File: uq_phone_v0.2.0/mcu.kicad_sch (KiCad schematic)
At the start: 23 parts, among them J6 Conn_ARM_SWD_TagConnect_TC2030, U5 TXB0108YZPR2, U6 STM32H733VGHx, U7 TXB0108YZPR2

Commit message: New Layout
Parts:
- removed R21: 4.7k, Resistor_SMD:R_0201_0603Metric, symbol Resistors:Resistor_4k7
- removed U5: TXB0108YZPR2, TXB0108YZPR2:YZP20, symbol TXB0108YZPR2:TXB0108YZPR2
- added C50, C51: 100nF, Capacitor_SMD:C_0201_0603Metric, symbol Capacitors:capacitor_100nF
- added J7, J9: 559092474, 559092474:CON_559092474, symbol 559092474:559092474
- added Q1, Q2: MMBT3904LP-7, MMBT3904LP-7:DFN101X61X53-3N, symbol MMBT3904LP-7:MMBT3904LP-7
- added R16, R17, R4: 4.7k, Resistor_SMD:R_0201_0603Metric, symbol Resistors:Resistor_4k7
- added R18, R19: 47k, Resistor_SMD:R_0201_0603Metric, symbol Resistors:Resistor_47k
- added U16: TXB0108YZPR2, TXB0108YZPR2:YZP20, symbol TXB0108YZPR2:TXB0108YZPR2
- added U5: TCA9509MRVHR, TCA9509MRVHR:RVH8_0P4X0P4, symbol TCA9509MRVHR:TCA9509MRVHR
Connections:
- net +1.8V: now also C50.1, J7.10, J7.11, J7.12, J7.9, U16.C4 (VCCA), U16.D4 (OE), U5.1 (VCCA), U5.5 (EN)
- net +3.3V: now also C51.1, R4.2, U16.C1 (VCCB), U5.8 (VCCB)
- net AUD_SCL: now also U5.2 (SCLA); no longer U7.A4 (A2)
- net AUD_SDA: now also U5.3 (SDAA); no longer U7.A3 (A1)
- net GND: now also C50.2, C51.2, J7.13, J7.14, J7.15, J7.16, J7.17, J7.18, J7.19, J7.20, J7.21, J7.22, J7.23, J7.24, J7.P1, J7.P2, J7.P3, J7.P4, Q1.2, Q2.2, R18.1, R19.1, U16.D1 (GND), U5.4 (GND), U5.9 (EPAD)
- net MCU_CTS: now also U16.E1 (B6)
- net MCU_DCD: now also U16.A1 (B2)
- net MCU_DSR: now also U16.A2 (B1)
- net MCU_DTR: now also U16.B2 (B3)
- net MCU_RI: now also U16.E2 (B8)
- net MCU_RTS: now also U16.D2 (B7)
- net MCU_RXD: now also U16.B1 (B4)
- net MCU_TXD: now also U16.C2 (B5)
- net MOB_CTS: now also U16.E4 (A6)
- net MOB_DCD: now also U16.A4 (A2)
- net MOB_DSR: now also U16.A3 (A1)
- net MOB_DTR: now also U16.B3 (A3)
- net MOB_PWR_CTL: now also R16.2
- net MOB_RI: now also U16.E3 (A8)
- net MOB_RST_CTL: now also R17.2
- net MOB_RTS: now also U16.D3 (A7)
- net MOB_RXD: now also U16.B4 (A4)
- net MOB_TXD: now also U16.C3 (A5)
- net SCL: now also R22.1, U5.7 (SCLB); no longer U7.A1 (B2)
- net SDA: now also R4.1, U5.6 (SDAB); no longer R22.1, U7.A2 (B1)
- new net: Q1.1, R16.1, R18.2
- new net: Q2.1, R17.1, R19.2
- new net MOB_PWR: Q1.3
- new net MOB_RST: Q2.3
- new net VBAT: J7.1, J7.2, J7.3, J7.4, J7.5, J7.6, J7.7, J7.8
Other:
- moved on the sheet: C14, C15, C16, C17, C18, C19, C20, C21, C22, C23, C24, C25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

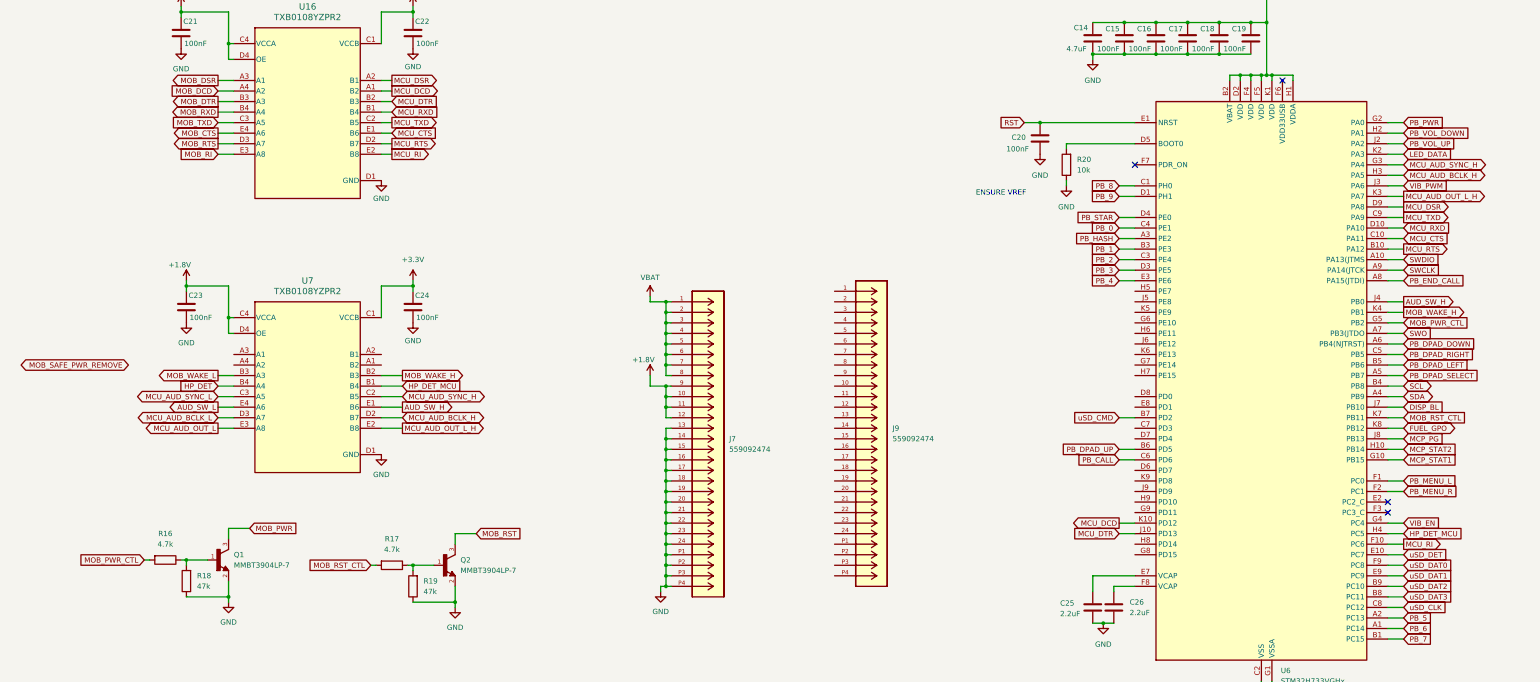
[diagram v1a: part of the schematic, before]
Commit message: Several Hours of Routing
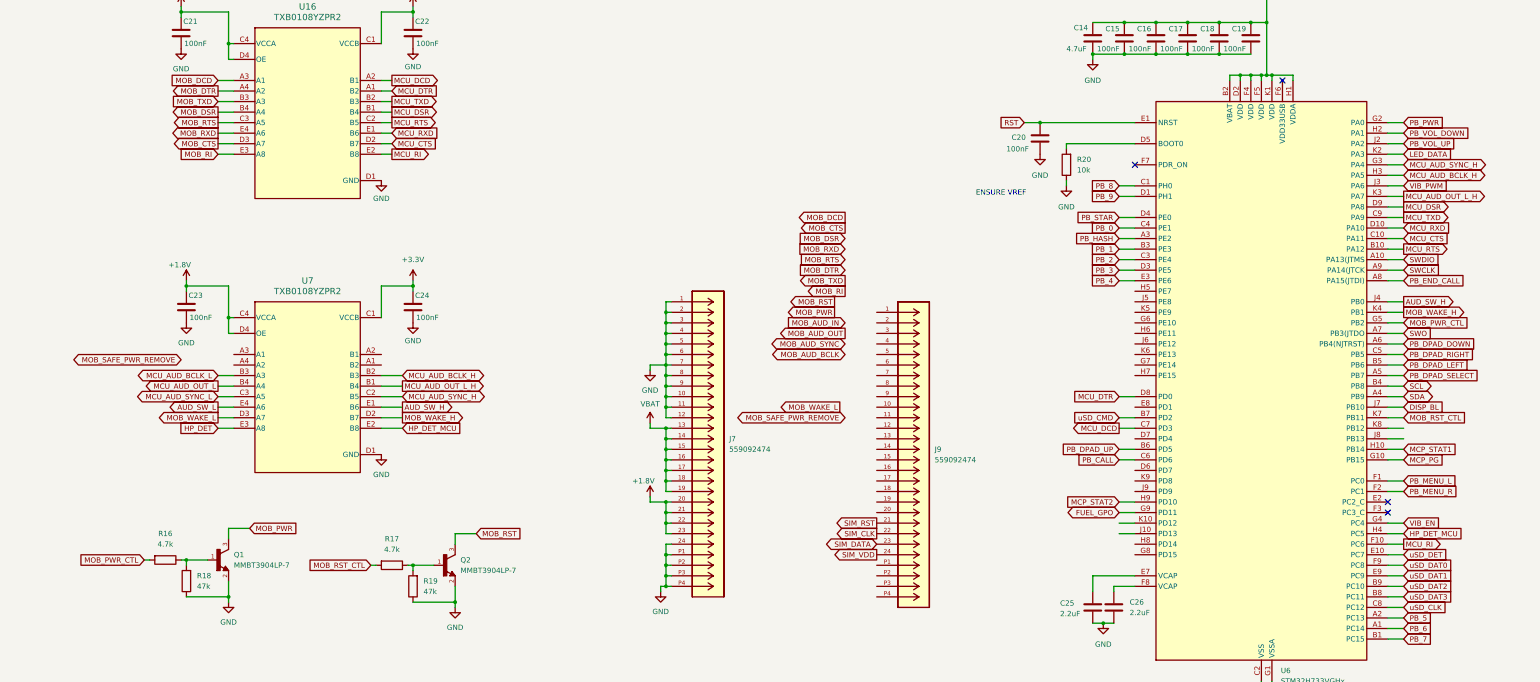
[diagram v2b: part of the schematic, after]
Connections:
- net +1.8V: now also J7.20, J7.21, J7.22, J7.23; no longer J7.10, J7.11, J7.12, J7.9
- net FUEL_GPO: now also U6.G9 (PD11); no longer U6.K8 (PB12)
- net GND: now also J7.1, J7.10, J7.11, J7.12, J7.2, J7.3, J7.4, J7.5, J7.6, J7.7, J7.8, J7.9; no longer J7.13, J7.14, J7.15, J7.16, J7.17, J7.18, J7.19, J7.20, J7.21, J7.22, J7.23
- net HP_DET: now also U7.E3 (A8); no longer U7.B4 (A4)
- net HP_DET_MCU: now also U7.E2 (B8); no longer U7.B1 (B4)
- net MCP_PG: now also U6.G10 (PB15); no longer U6.J8 (PB13)
- net MCP_STAT1: now also U6.H10 (PB14); no longer U6.G10 (PB15)
- net MCP_STAT2: now also U6.H9 (PD10); no longer U6.H10 (PB14)
- net MCU_AUD_BCLK_H: now also U7.B2 (B3); no longer U7.D2 (B7)
- net MCU_AUD_BCLK_L: now also U7.B3 (A3); no longer U7.D3 (A7)
- net MCU_AUD_OUT_L: now also U7.B4 (A4); no longer U7.E3 (A8)
- net MCU_AUD_OUT_L_H: now also U7.B1 (B4); no longer U7.E2 (B8)
- net MCU_CTS: now also U16.D2 (B7); no longer U16.E1 (B6)
- net MCU_DCD: now also U16.A2 (B1), U6.C7 (PD3); no longer U16.A1 (B2), U6.K10 (PD12)
- net MCU_DSR: now also U16.B1 (B4); no longer U16.A2 (B1)
- net MCU_DTR: now also U16.A1 (B2), U6.D8 (PD0); no longer U16.B2 (B3), U6.J10 (PD13)
- net MCU_RTS: now also U16.C2 (B5); no longer U16.D2 (B7)
- net MCU_RXD: now also U16.E1 (B6); no longer U16.B1 (B4)
- net MCU_TXD: now also U16.B2 (B3); no longer U16.C2 (B5)
- net MOB_CTS: now also U16.D3 (A7); no longer U16.E4 (A6)
- net MOB_DCD: now also U16.A3 (A1); no longer U16.A4 (A2)
- net MOB_DSR: now also U16.B4 (A4); no longer U16.A3 (A1)
- net MOB_DTR: now also U16.A4 (A2); no longer U16.B3 (A3)
- net MOB_RTS: now also U16.C3 (A5); no longer U16.D3 (A7)
- net MOB_RXD: now also U16.E4 (A6); no longer U16.B4 (A4)
- net MOB_TXD: now also U16.B3 (A3); no longer U16.C3 (A5)
- net MOB_WAKE_H: now also U7.D2 (B7); no longer U7.B2 (B3)
- net MOB_WAKE_L: now also U7.D3 (A7); no longer U7.B3 (A3)
- net VBAT: now also J7.13, J7.14, J7.15, J7.16, J7.17, J7.18, J7.19; no longer J7.1, J7.2, J7.3, J7.4, J7.5, J7.6, J7.7, J7.8
- net SIM_RST: now reaches J9.21
- net SIM_CLK: now reaches J9.22
- net SIM_DATA: now reaches J9.23
- net SIM_VDD: now reaches J9.24
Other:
- moved on the sheet: J9

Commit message: More routing and placements
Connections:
- net AUD_SW_H: now also U6.K10 (PD12); no longer U6.J4 (PB0)
- net HP_DET_MCU: now also U6.J10 (PD13); no longer U6.H4 (PC5)
- net MOB_AUD_BCLK: now also J9.9
- net MOB_AUD_IN: now also J9.10
- net MOB_AUD_OUT: now also J9.11
- net MOB_AUD_SYNC: now also J9.12
- net MOB_CTS: now also J9.18
- net MOB_DCD: now also J9.13
- net MOB_DSR: now also J9.15
- net MOB_DTR: now also J9.14
- net MOB_PWR: now also J9.1
- net MOB_PWR_CTL: now also U6.A2 (PC13); no longer U6.G5 (PB2)
- net MOB_RI: now also J9.20
- net MOB_RST: now also J9.2
- net MOB_RST_CTL: now also U6.A1 (PC14); no longer U6.K7 (PB11)
- net MOB_RTS: now also J9.17
- net MOB_RXD: now also J9.19
- net MOB_TXD: now also J9.16
- net MOB_WAKE_H: now also U6.K9 (PD8); no longer U6.K4 (PB1)
- net MOB_WAKE_L: now also J9.4
- net PB_5: now also U6.K7 (PB11); no longer U6.A2 (PC13)
- net PB_6: now also U6.K8 (PB12); no longer U6.A1 (PC14)
- net MOB_SAFE_PWR_REMOVE_L: now reaches J9.3
- net MOB_SAFE_PWR_REMOVE_L: now also U7.A4 (A2)
- net MOB_SAFE_PWR_REMOVE_H: now reaches U6.J9 (PD9)
- net MOB_SAFE_PWR_REMOVE_H: now also U7.A1 (B2)
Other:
- note added: "Mezzanine Connectors"
- moved on the sheet: C21, C22, C23, C24, C50, C51, J6, J7, J9, Q1, Q2, R16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
